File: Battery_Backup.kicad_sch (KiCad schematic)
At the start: 0 parts

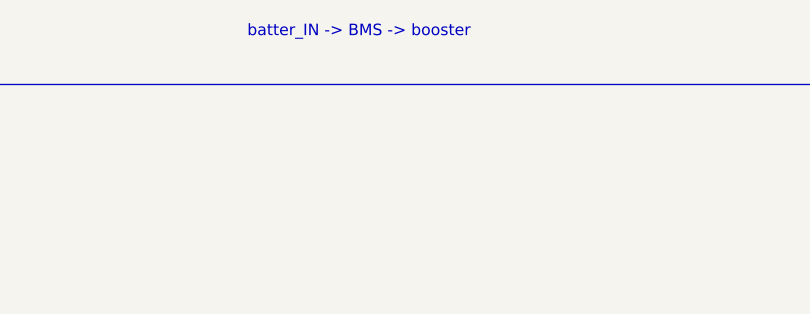
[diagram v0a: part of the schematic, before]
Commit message: Schematic Completed
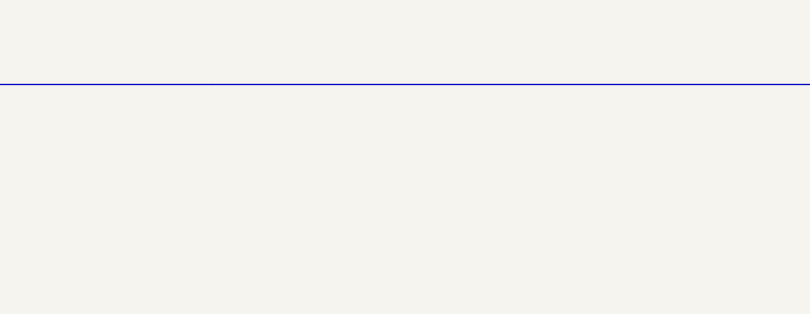
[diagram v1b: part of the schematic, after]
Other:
- note removed: "batter_IN -> BMS -> booster"
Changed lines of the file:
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@@
     (stroke (width 0) (type default))
   )
-  (text "batter_IN -> BMS -> booster" (at 88.9 7.62 0)
-    (effects (font (size 1.27 1.27)) (justify left bottom))
-  )
 )
